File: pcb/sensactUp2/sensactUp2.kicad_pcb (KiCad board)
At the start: 2 copper layers, 71 x 71 mm, 73 parts, among them IC1 MD8002A, J1 PROG, J2 GND CL CH 24V, J3 GND SCL SDA 3V3, J4 GND EXT1...EXT16 1W, J5 24V CH CL GND, J6 EXT 11...7, J7 SPK, Q3 Q_NPN_BEC, SW1 RotEnc, SW2 Reset, SW3 UserButton, SW4 TERM, U1 ESP32, U2 TPS5430DDA, U3 DS2482, U4 SN65HVD230, U5 AP1117-33, U6 PCA9555PW, X1 Display_LH154K-PG04

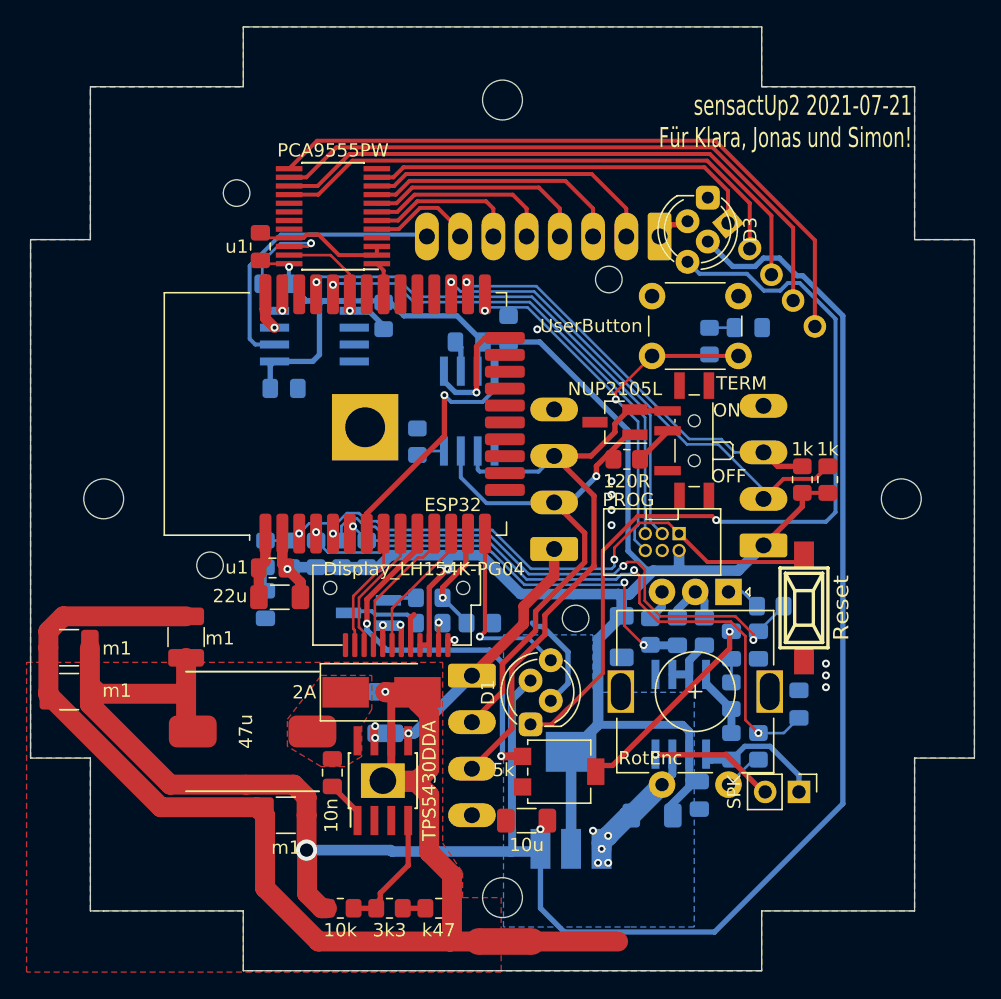
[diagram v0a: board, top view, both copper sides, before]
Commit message: sensactUP3 and sensactUPUpdates to KiCad6
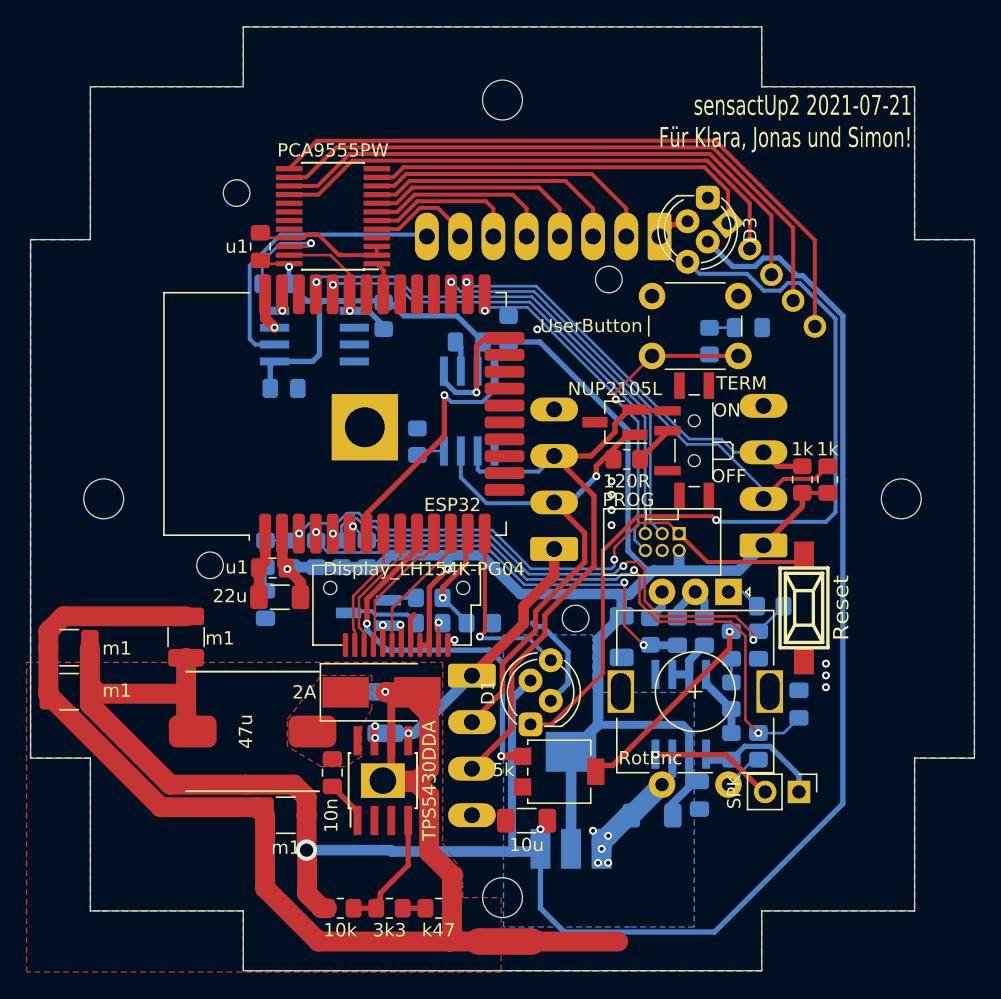
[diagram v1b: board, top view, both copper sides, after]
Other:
- net class Default removed
- net class HighVoltage removed
